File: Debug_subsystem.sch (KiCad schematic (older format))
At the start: 2 parts, among them J501 Conn_ARM_JTAG_SWD_10, J502 3.3V

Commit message: Recovered the .lib for flash symbol. Relinked in schematic
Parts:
- J501: symbol Connector:Conn_ARM_JTAG_SWD_10 -> BeagleBone-Black-Cape-rescue:Conn_ARM_JTAG_SWD_10-Connector
- J502: symbol Connector:Conn_01x03_Female -> BeagleBone-Black-Cape-rescue:Conn_01x03_Female-Connector
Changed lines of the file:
@@
 $EndDescr
 $Comp
-L Connector:Conn_ARM_JTAG_SWD_10 J501
+L BeagleBone-Black-Cape-rescue:Conn_ARM_JTAG_SWD_10-Connector J501
 U 1 1 614AA0C1
 P 5150 3550
@@
 MCU_RESET
 $Comp
-L power:GND #PWR0501
+L BeagleBone-Black-Cape-rescue:GND-power #PWR0501
 U 1 1 614AB0A8
 P 5100 4200
@@
 MCU_VDD
 $Comp
-L Connector:Conn_01x03_Female J502
+L BeagleBone-Black-Cape-rescue:Conn_01x03_Female-Connector J502
 U 1 1 614ABF85
 P 7550 3550
@@
 MCU_VDD
 $Comp
-L power:GND #PWR0502
+L BeagleBone-Black-Cape-rescue:GND-power #PWR0502
 U 1 1 614AC7F9
 P 7150 3800

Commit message: lib update so it only includes user-made library
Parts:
- J501: symbol BeagleBone-Black-Cape-rescue:Conn_ARM_JTAG_SWD_10-Connector -> UserMade-BB-Zigbee-Gateway-CAPE:Conn_ARM_JTAG_SWD_10-Connector
- J502: symbol BeagleBone-Black-Cape-rescue:Conn_01x03_Female-Connector -> UserMade-BB-Zigbee-Gateway-CAPE:Conn_01x03_Female-Connector
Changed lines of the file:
@@
 $EndDescr
 $Comp
-L BeagleBone-Black-Cape-rescue:Conn_ARM_JTAG_SWD_10-Connector J501
+L UserMade-BB-Zigbee-Gateway-CAPE:Conn_ARM_JTAG_SWD_10-Connector J501
 U 1 1 614AA0C1
 P 5150 3550
@@
 MCU_RESET
 $Comp
-L BeagleBone-Black-Cape-rescue:GND-power #PWR0501
+L UserMade-BB-Zigbee-Gateway-CAPE:GND-power #PWR0501
 U 1 1 614AB0A8
 P 5100 4200
@@
 MCU_VDD
 $Comp
-L BeagleBone-Black-Cape-rescue:Conn_01x03_Female-Connector J502
+L UserMade-BB-Zigbee-Gateway-CAPE:Conn_01x03_Female-Connector J502
 U 1 1 614ABF85
 P 7550 3550
@@
 MCU_VDD
 $Comp
-L BeagleBone-Black-Cape-rescue:GND-power #PWR0502
+L UserMade-BB-Zigbee-Gateway-CAPE:GND-power #PWR0502
 U 1 1 614AC7F9
 P 7150 3800

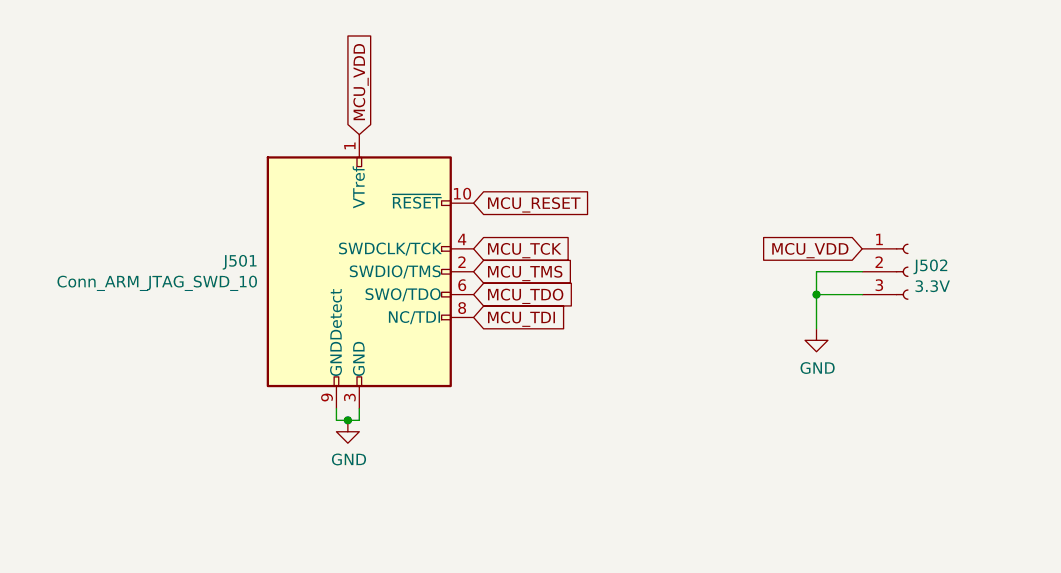
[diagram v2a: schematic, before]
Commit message: final edits before it'll be untouched
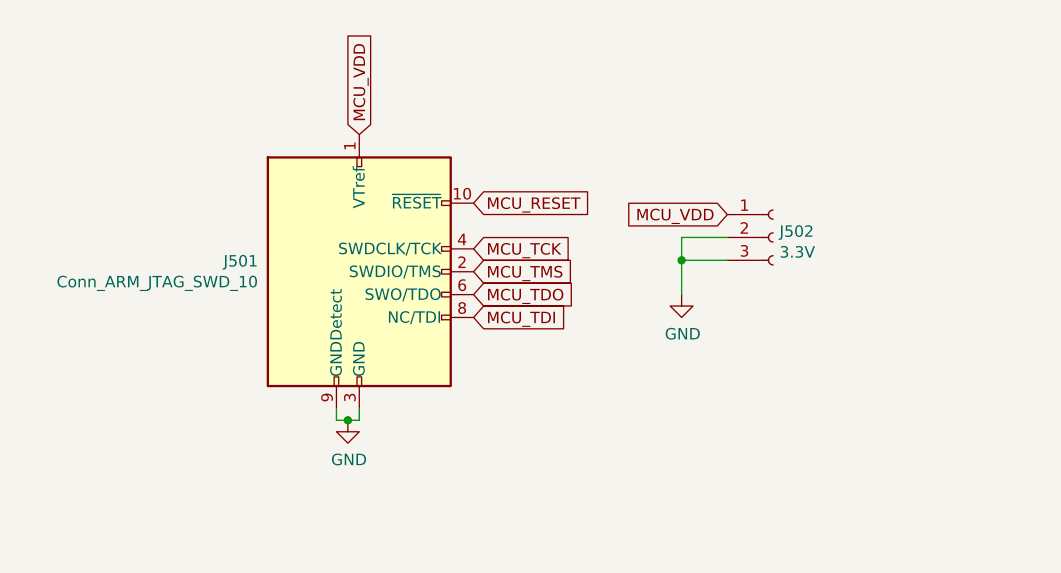
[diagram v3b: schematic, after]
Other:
- moved on the sheet: J502
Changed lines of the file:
@@
 L UserMade-BB-Zigbee-Gateway-CAPE:Conn_01x03_Female-Connector J502
 U 1 1 614ABF85
-P 7550 3550
-F 0 "J502" H 7578 3576 50  0000 L CNN
-F 1 "3.3V" H 7578 3485 50  0000 L CNN
-F 2 "Connector_PinHeader_2.54mm:PinHeader_1x03_P2.54mm_Vertical" H 7550 3550 50  0001 C CNN
-F 3 "~" H 7550 3550 50  0001 C CNN
-	1    7550 3550
+P 6960 3400
+F 0 "J502" H 6988 3426 50  0000 L CNN
+F 1 "3.3V" H 6988 3335 50  0000 L CNN
+F 2 "Connector_PinHeader_2.54mm:PinHeader_1x03_P2.54mm_Vertical" H 6960 3400 50  0001 C CNN
+F 3 "~" H 6960 3400 50  0001 C CNN
+	1    6960 3400
 	1    0    0    -1
 $EndComp
-Text GLabel 7350 3450 0    50   Input ~ 0
+Text GLabel 6760 3300 0    50   Input ~ 0
 MCU_VDD
 $Comp
 L UserMade-BB-Zigbee-Gateway-CAPE:GND-power #PWR0502
 U 1 1 614AC7F9
-P 7150 3800
-F 0 "#PWR0502" H 7150 3550 50  0001 C CNN
-F 1 "GND" H 7155 3627 50  0000 C CNN
-F 2 "" H 7150 3800 50  0001 C CNN
-F 3 "" H 7150 3800 50  0001 C CNN
-	1    7150 3800
+P 6560 3650
+F 0 "#PWR0502" H 6560 3400 50  0001 C CNN
+F 1 "GND" H 6565 3477 50  0000 C CNN
+F 2 "" H 6560 3650 50  0001 C CNN
+F 3 "" H 6560 3650 50  0001 C CNN
+	1    6560 3650
 	1    0    0    -1
 $EndComp
 Wire Wire Line
-	7150 3800 7150 3650
+	6560 3650 6560 3500
 Wire Wire Line
-	7150 3550 7350 3550
+	6560 3400 6760 3400
 Wire Wire Line
-	7350 3650 7150 3650
-Connection ~ 7150 3650
+	6760 3500 6560 3500
+Connection ~ 6560 3500
 Wire Wire Line
-	7150 3650 7150 3550
+	6560 3500 6560 3400
 $EndSCHEMATC
